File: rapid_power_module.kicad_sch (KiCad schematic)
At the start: 206 parts, among them J1 Conn_02x04_Top_Bottom, J10 JST-GH 4Pin, J11 SWD Header, J12 SWD Header, J16 USB_C_Receptacle_USB2.0, J17 TC2050, J2 Conn_02x03_Odd_Even, J3 Conn_02x04_Top_Bottom, J4 Conn_02x03_Odd_Even, J5 Molex MicroFit 2x2, J6 Molex MicroFit 2x2, J7 Molex MicroFit 2x2, J8 Molex MicroFit 2x2, Q1 AOSP21321, Q12 AOSP21321, Q2 AOSP21321, Q3 AOSP21321, Q4 HiDRV1, Q5 LoDRV1, Q6 HiDRV2, Q7 LoDRV2, SW1 KMR721NGLFS, SW2 KMR721NGLFS, U1 BQ25756RRVR, U10 L7805, U11 MCP2562-E-SN, U12 STM32F105RCTx, U13 AZ1117I-3.3, U14 TPD4E1U06, U15 TPD4E1U06, U2 CYPD3177-24LQ, U3 BQ76952PFBR, Y3 8MHz 12pF

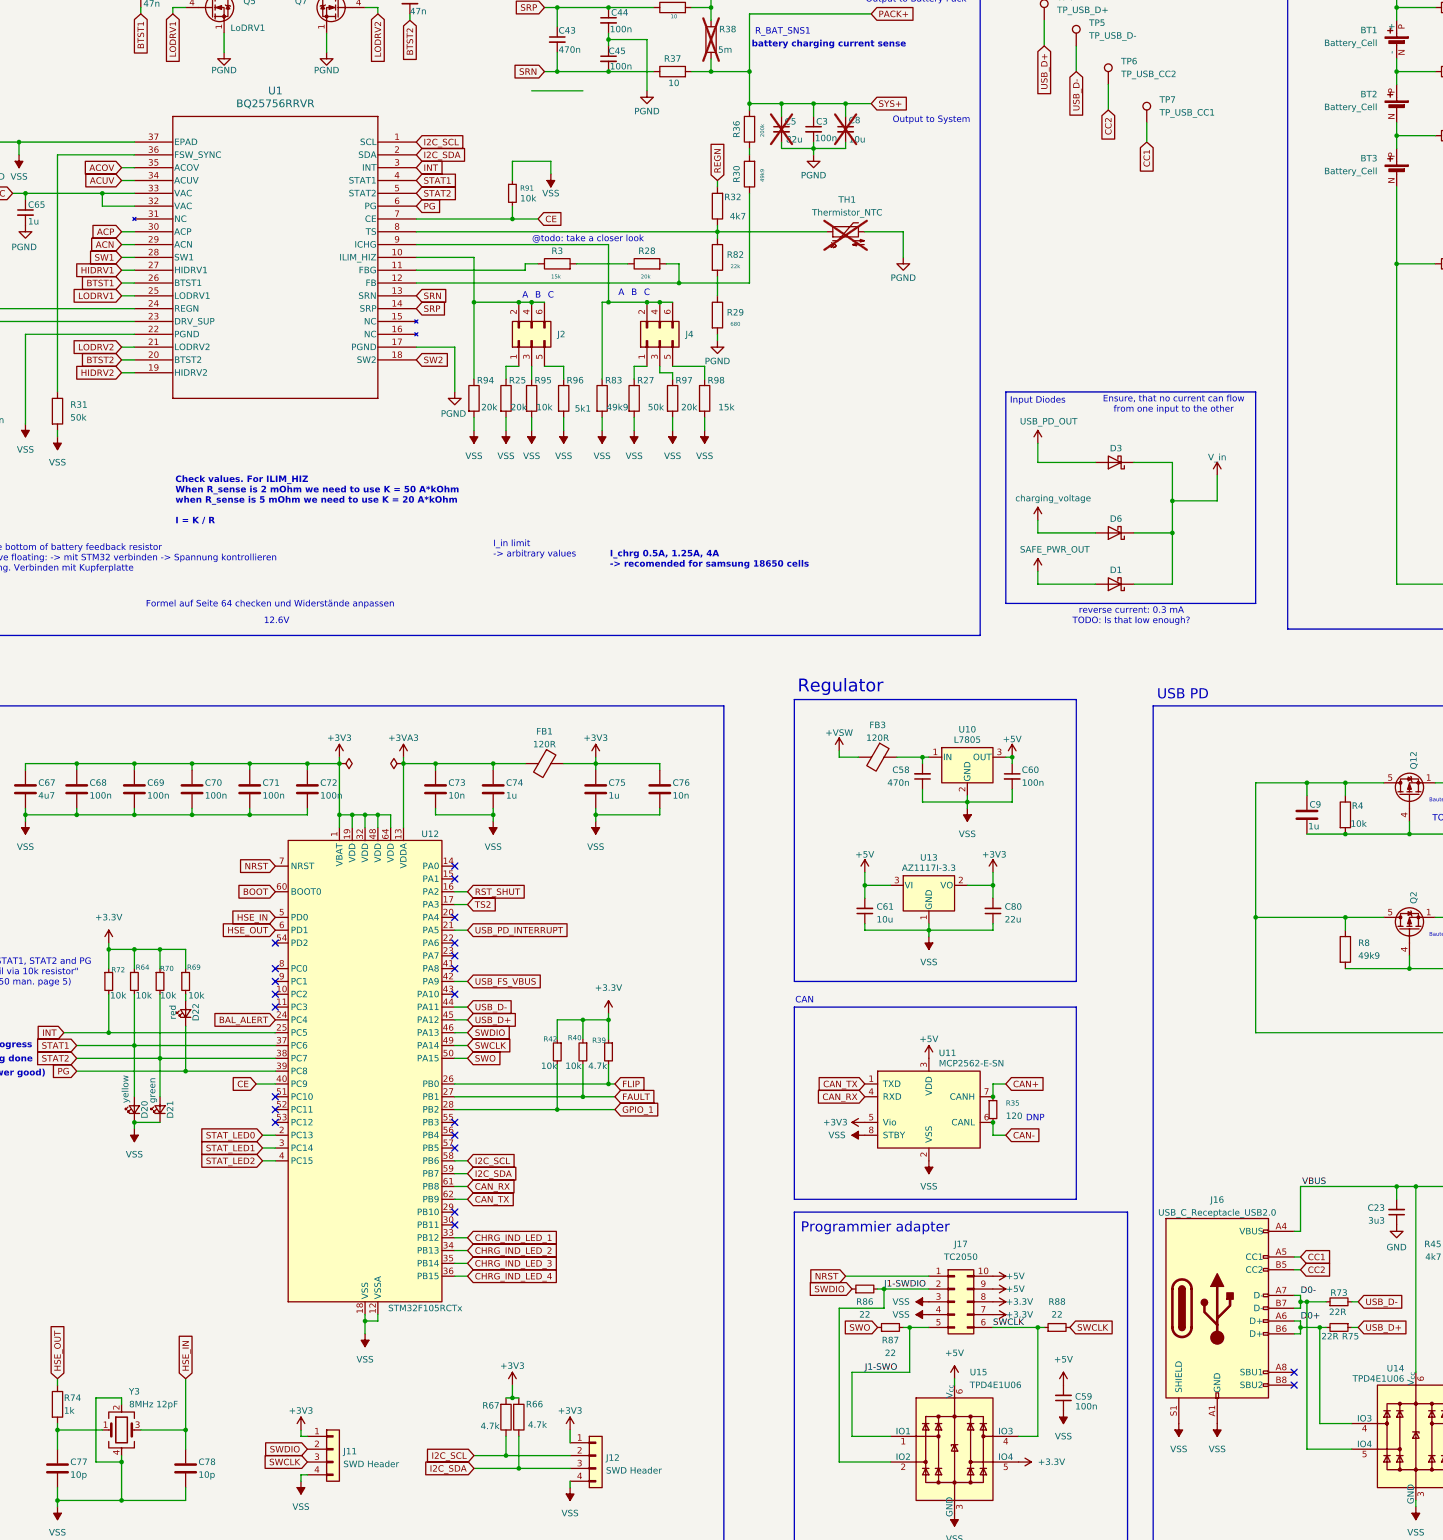
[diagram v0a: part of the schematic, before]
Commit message: more routing work
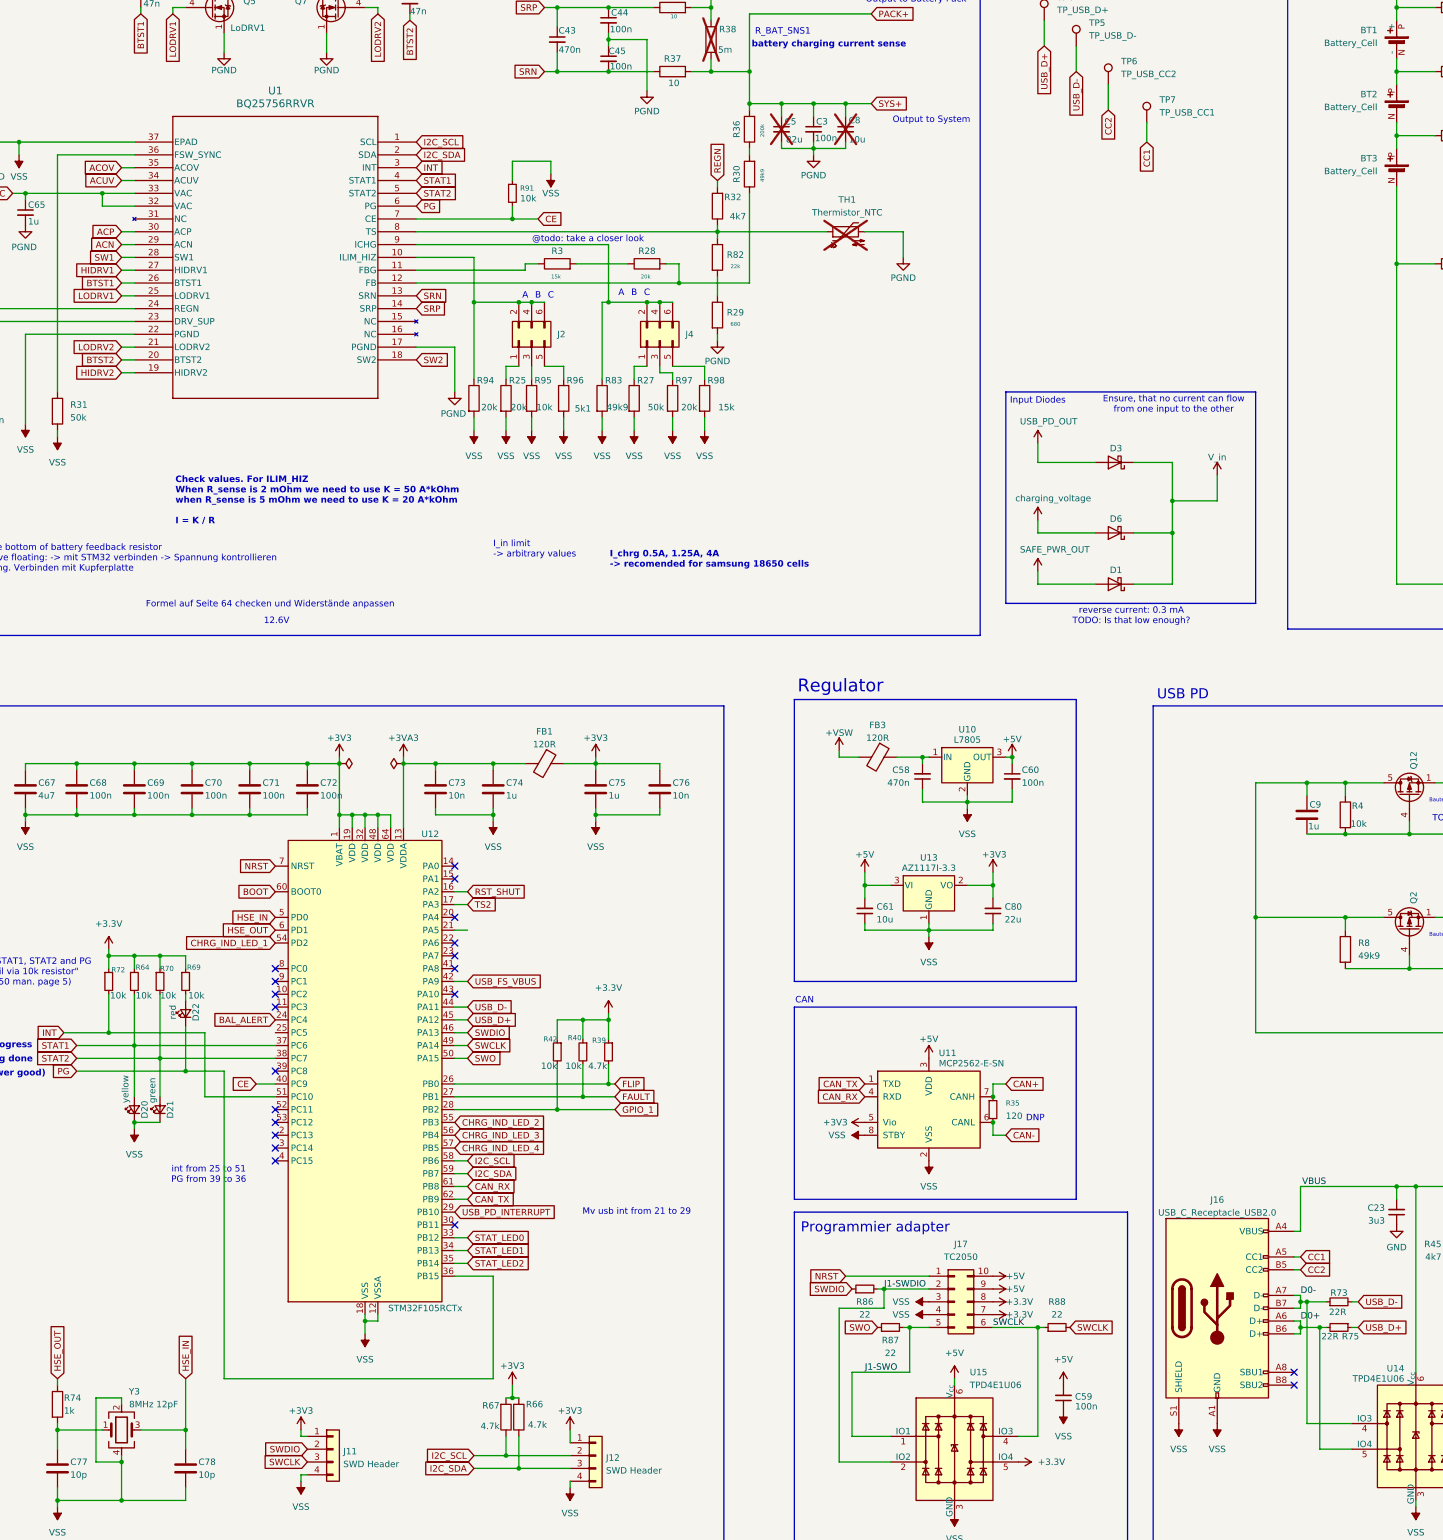
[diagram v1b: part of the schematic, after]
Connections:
- net CHRG_IND_LED_1: now also U12.54 (PD2); no longer U12.33 (PB12)
- net CHRG_IND_LED_2: now also U12.55 (PB3); no longer U12.34 (PB13)
- net CHRG_IND_LED_3: now also U12.56 (PB4); no longer U12.35 (PB14)
- net CHRG_IND_LED_4: now also U12.57 (PB5); no longer U12.36 (PB15)
- net D0+: now also U14.5 (IO4); no longer U14.4 (IO3)
- net D0-: now also U14.4 (IO3); no longer U14.5 (IO4)
- net INT: now also U12.51 (PC10); no longer U12.25 (PC5)
- net PG: now also U12.36 (PB15); no longer U12.39 (PC8)
- net STAT_LED0: now also U12.33 (PB12); no longer U12.2 (PC13)
- net STAT_LED1: now also U12.34 (PB13); no longer U12.3 (PC14)
- net STAT_LED2: now also U12.35 (PB14); no longer U12.4 (PC15)
- net USB_PD_INTERRUPT: now also U12.29 (PB10); no longer U12.21 (PA5)
- no-connect marks 35 -> 33
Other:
- note added: "Mv usb int from 21 to 29"
- note added: "int from 25 to 51 PG from 39 to 36"

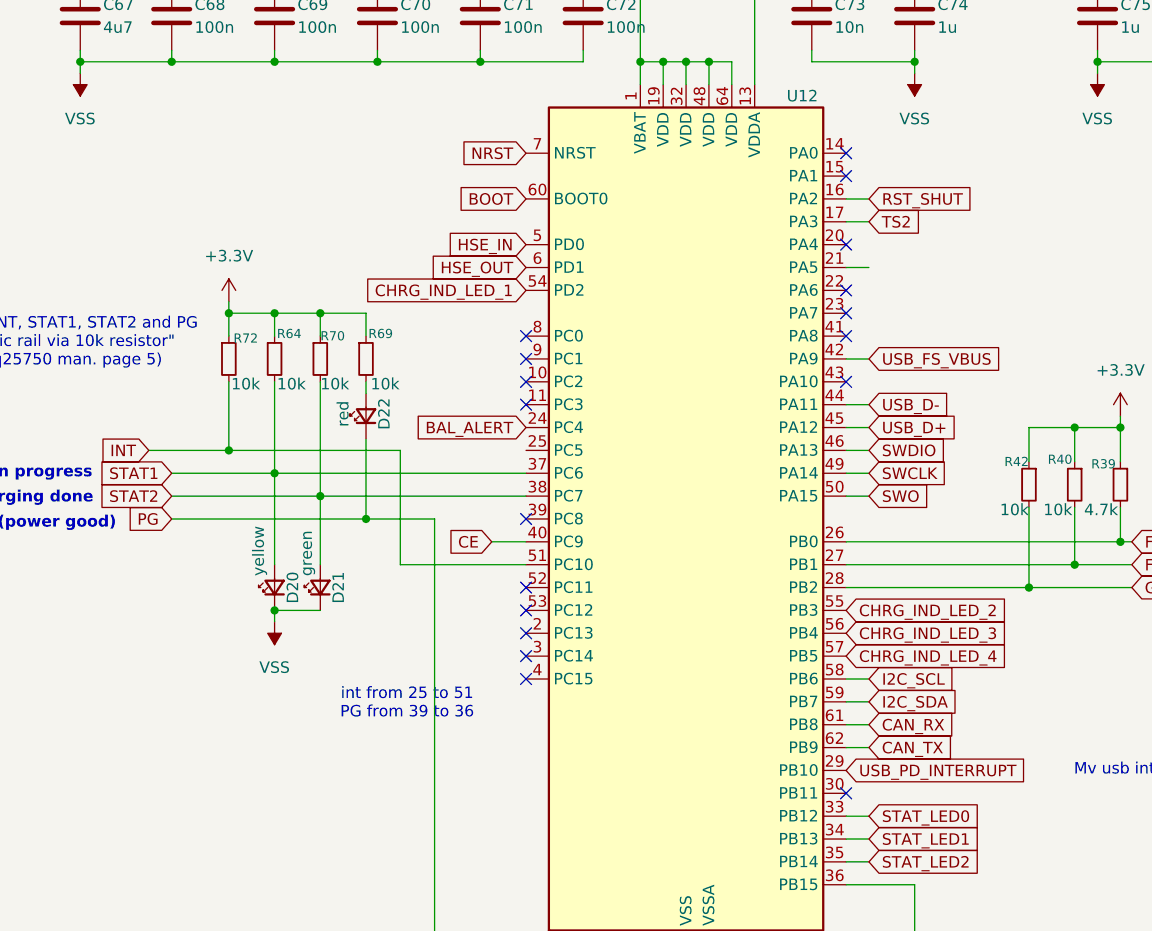
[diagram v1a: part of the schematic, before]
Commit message: more routing
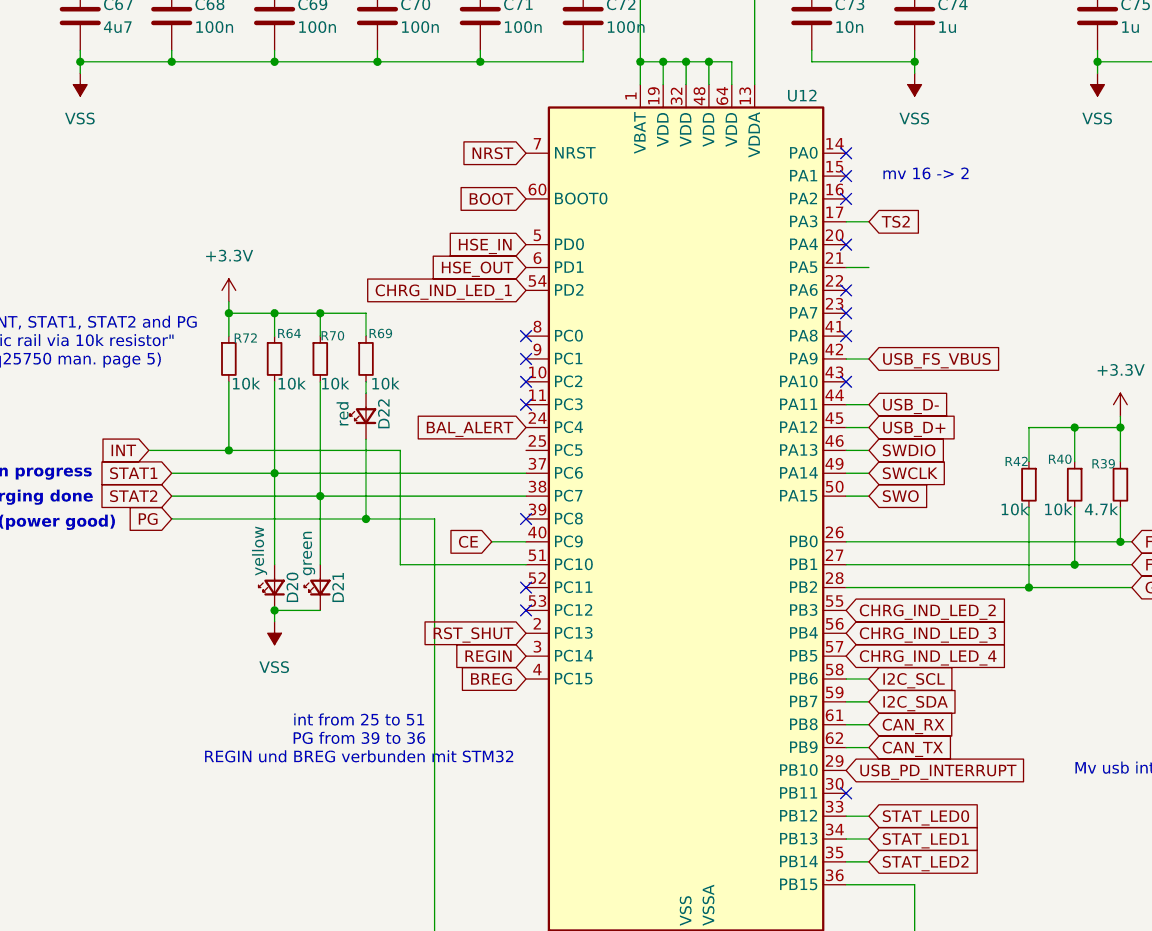
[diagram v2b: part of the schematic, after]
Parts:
- D4: footprint Package_TO_SOT_THT:TO-220-3_Vertical -> Diode_SMD:D_SOD-323; LCSC C5358933 -> C191023
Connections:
- net BREG: now also U12.4 (PC15)
- net REGIN: now also U12.3 (PC14)
- net RST_SHUT: now also U12.2 (PC13); no longer U12.16 (PA2)
- no-connect marks 33 -> 31
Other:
- note added: "int from 25 to 51 PG from 39 to 36 REGIN und BREG verbunden mit STM32"
- note added: "mv 16 -> 2"
- note removed: "int from 25 to 51 PG from 39 to 36"
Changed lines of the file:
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@@
 		)
 	)
-	(text "int from 25 to 51\nPG from 39 to 36"
+	(text "int from 25 to 51\nPG from 39 to 36\nREGIN und BREG verbunden mit STM32"
 		(exclude_from_sim no)
-		(at 113.792 326.644 0)
+		(at 108.458 330.708 0)
 		(effects
 			(font
@@
 		)
 	)
+	(text "mv 16 -> 2"
+		(exclude_from_sim no)
+		(at 171.45 267.97 0)
+		(effects
+			(font
+				(size 1.27 1.27)
+			)
+		)
+	)
 	(text "@todo: take a closer look"
 		(exclude_from_sim no)
@@
 	)
 	(no_connect
-		(at 127 323.85)
-	)
-	(no_connect
 		(at 488.95 130.81)
 	)
@@
 	)
 	(no_connect
+		(at 162.56 270.51)
+	)
+	(no_connect
 		(at 488.95 123.19)
 	)
@@
 	)
 	(no_connect
-		(at 127 318.77)
-	)
-	(no_connect
-		(at 127 321.31)
-	)
-	(no_connect
 		(at 488.95 110.49)
 	)
@@
 	(wire
 		(pts
-			(xy 165.1 270.51) (xy 162.56 270.51)
-		)
-		(stroke
-			(width 0)
-			(type default)
-		)
-	)
-	(wire
-		(pts
 			(xy 205.74 167.64) (xy 203.2 167.64)
 		)
@@
 	(global_label "RST_SHUT"
 		(shape input)
-		(at 165.1 270.51 0)
+		(at 127 318.77 180)
 		(fields_autoplaced yes)
 		(effects
@@
 				(size 1.27 1.27)
 			)
-			(justify left)
+			(justify right)
 		)
 		(property "Intersheetrefs" "${INTERSHEET_REFS}"
-			(at 177.338 270.51 0)
+			(at 114.762 318.77 0)
 			(effects
 				(font
 					(size 1.27 1.27)
 				)
-				(justify left)
+				(justify right)
 				(hide yes)
 			)
@@
 		)
 	)
+	(global_label "REGIN"
+		(shape input)
+		(at 127 321.31 180)
+		(fields_autoplaced yes)
+		(effects
+			(font
+				(size 1.27 1.27)
+			)
+			(justify right)
+		)
+		(property "Intersheetrefs" "${INTERSHEET_REFS}"
+			(at 118.3905 321.31 0)
+			(effects
+				(font
+					(size 1.27 1.27)
+				)
+				(justify right)
+				(hide yes)
+			)
+		)
+	)
 	(global_label "SWCLK"
 		(shape input)
@@
 		)
 	)
+	(global_label "BREG"
+		(shape input)
+		(at 127 323.85 180)
+		(fields_autoplaced yes)
+		(effects
+			(font
+				(size 1.27 1.27)
+			)
+			(justify right)
+		)
+		(property "Intersheetrefs" "${INTERSHEET_REFS}"
+			(at 119.0558 323.85 0)
+			(effects
+				(font
+					(size 1.27 1.27)
+				)
+				(justify right)
+				(hide yes)
+			)
+		)
+	)
 	(global_label "SWDIO"
 		(shape input)
@@
 			)
 		)
-		(property "Footprint" "Package_TO_SOT_THT:TO-220-3_Vertical"
+		(property "Footprint" "Diode_SMD:D_SOD-323"
 			(at 533.4 326.39 0)
 			(effects
@@
 			)
 		)
-		(property "LCSC" "C5358933"
+		(property "LCSC" "C191023"
 			(at 533.4 326.39 0)
 			(effects
